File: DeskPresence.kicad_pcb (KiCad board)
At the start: 2 copper layers, 26 x 36 mm, 1 part, among them J1 USB_A

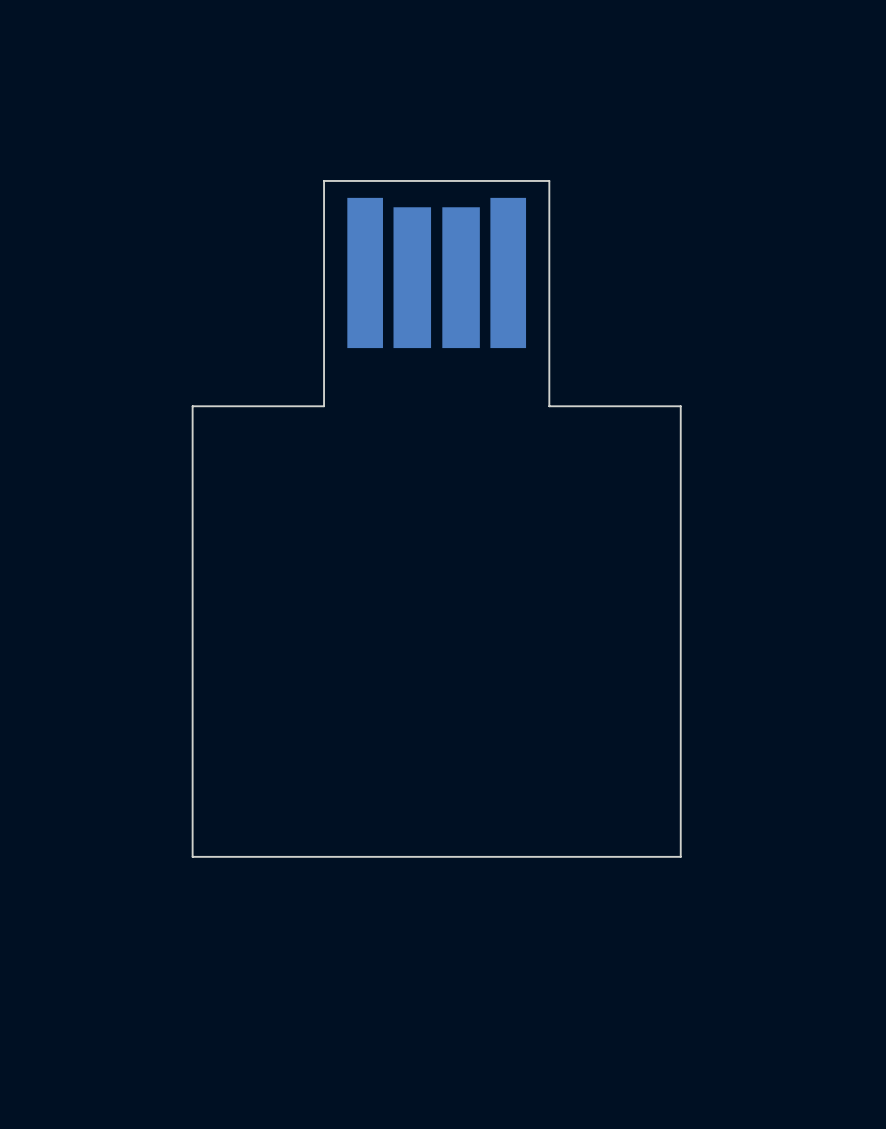
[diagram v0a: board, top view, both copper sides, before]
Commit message: Sketchy first pcb
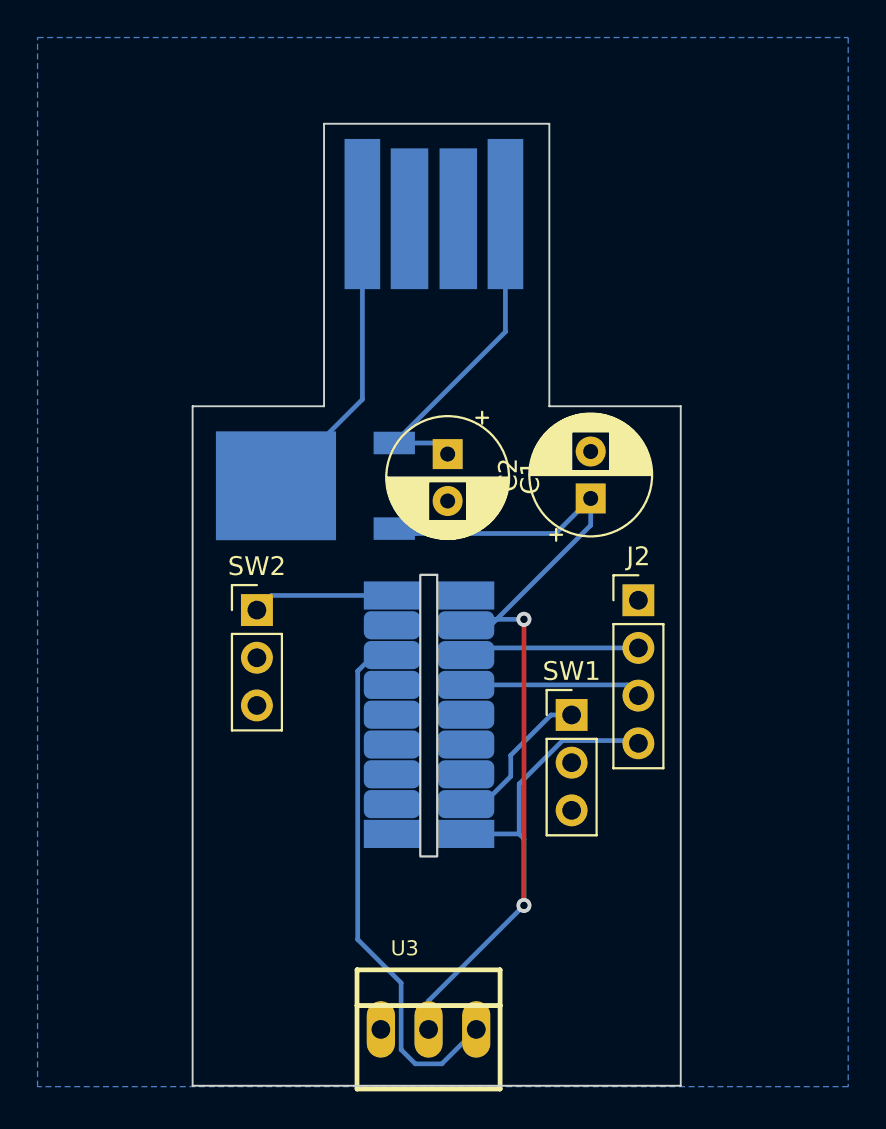
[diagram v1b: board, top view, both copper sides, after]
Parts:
- added C1: C_Polarized, Capacitor_THT:CP_Radial_D6.3mm_P2.50mm, F.Cu at (100.6, 108.5)
- added C2: C_Polarized, Capacitor_THT:CP_Radial_D6.3mm_P2.50mm, F.Cu at (108.2, 110.9)
- added J2: TTL, Connector_PinHeader_2.54mm:PinHeader_1x04_P2.54mm_Vertical, F.Cu at (110.7, 116.3)
- added SW1: MODE, Connector_PinHeader_2.54mm:PinHeader_1x03_P2.54mm_Vertical, F.Cu at (107.2, 122.4)
- added SW2: RESET, Connector_PinHeader_2.54mm:PinHeader_1x03_P2.54mm_Vertical, F.Cu at (90.4, 116.9)
- added U1: UA78M33_TO252, Package_TO_SOT_SMD:TO-252-2, B.Cu at (93.5, 110.2)
- added U2: esp-01m, esp-01m:esp-01m, B.Cu at (99.6, 122.4)
- added U3: GP2Y0A02YK0F, GP2Y0A02YK0F:GP2Y0A02YK0F, F.Cu at (99.6, 139.2)
- moved J1 16.3 mm to (99.9, 90.9)
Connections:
- J1 pad 1: unconnected-(J1-Pad1) -> +5V
- J1 pad 4: unconnected-(J1-Pad4) -> GND
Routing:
- net +3V3: track 0.00 -> 65.5 mm, vias 0 -> 2
- net /Data: track 0.00 -> 28.4 mm
- net +5V: track 0.00 -> 17.7 mm
- net GND: track 0.00 -> 16.4 mm
- net RX: track 0.00 -> 9.41 mm
- net TX: track 0.00 -> 9.33 mm
- net Net-(SW1-Pad1): track 0.00 -> 8.25 mm
- net Net-(SW2-Pad1): track 0.00 -> 7.52 mm
- added copper zone on B.Cu, net GND
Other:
- board size 26 x 36 mm -> 26 x 51.2 mm
